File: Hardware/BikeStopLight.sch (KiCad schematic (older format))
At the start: 63 parts, among them J1 ST-Link, J2 PWR, J3 BAT, J4 Conn_01x01, J5 Conn_01x01, J6 Conn_01x08, Q1 NTD4909N, U1 MCP1703A-3302_SOT23, U2 STM32L052K8Tx, U3 RFM95W-868S2, Y1 ABS07-120-32.768KHZ-T

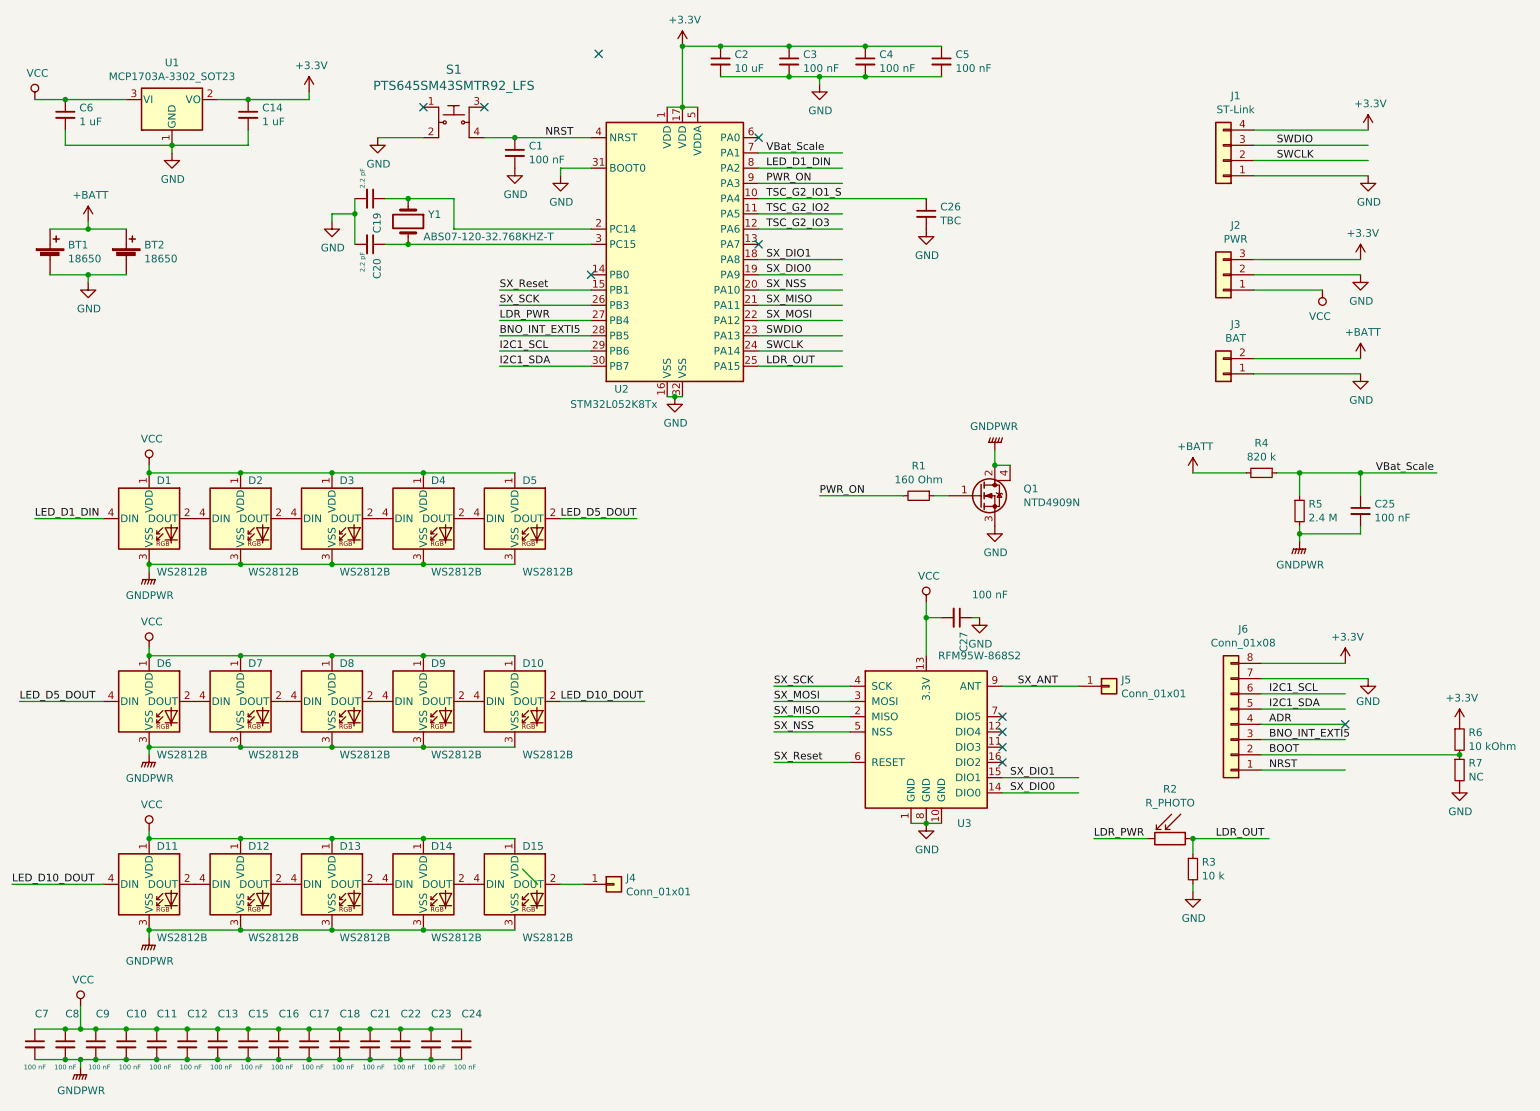
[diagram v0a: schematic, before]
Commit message: WIP - Routed
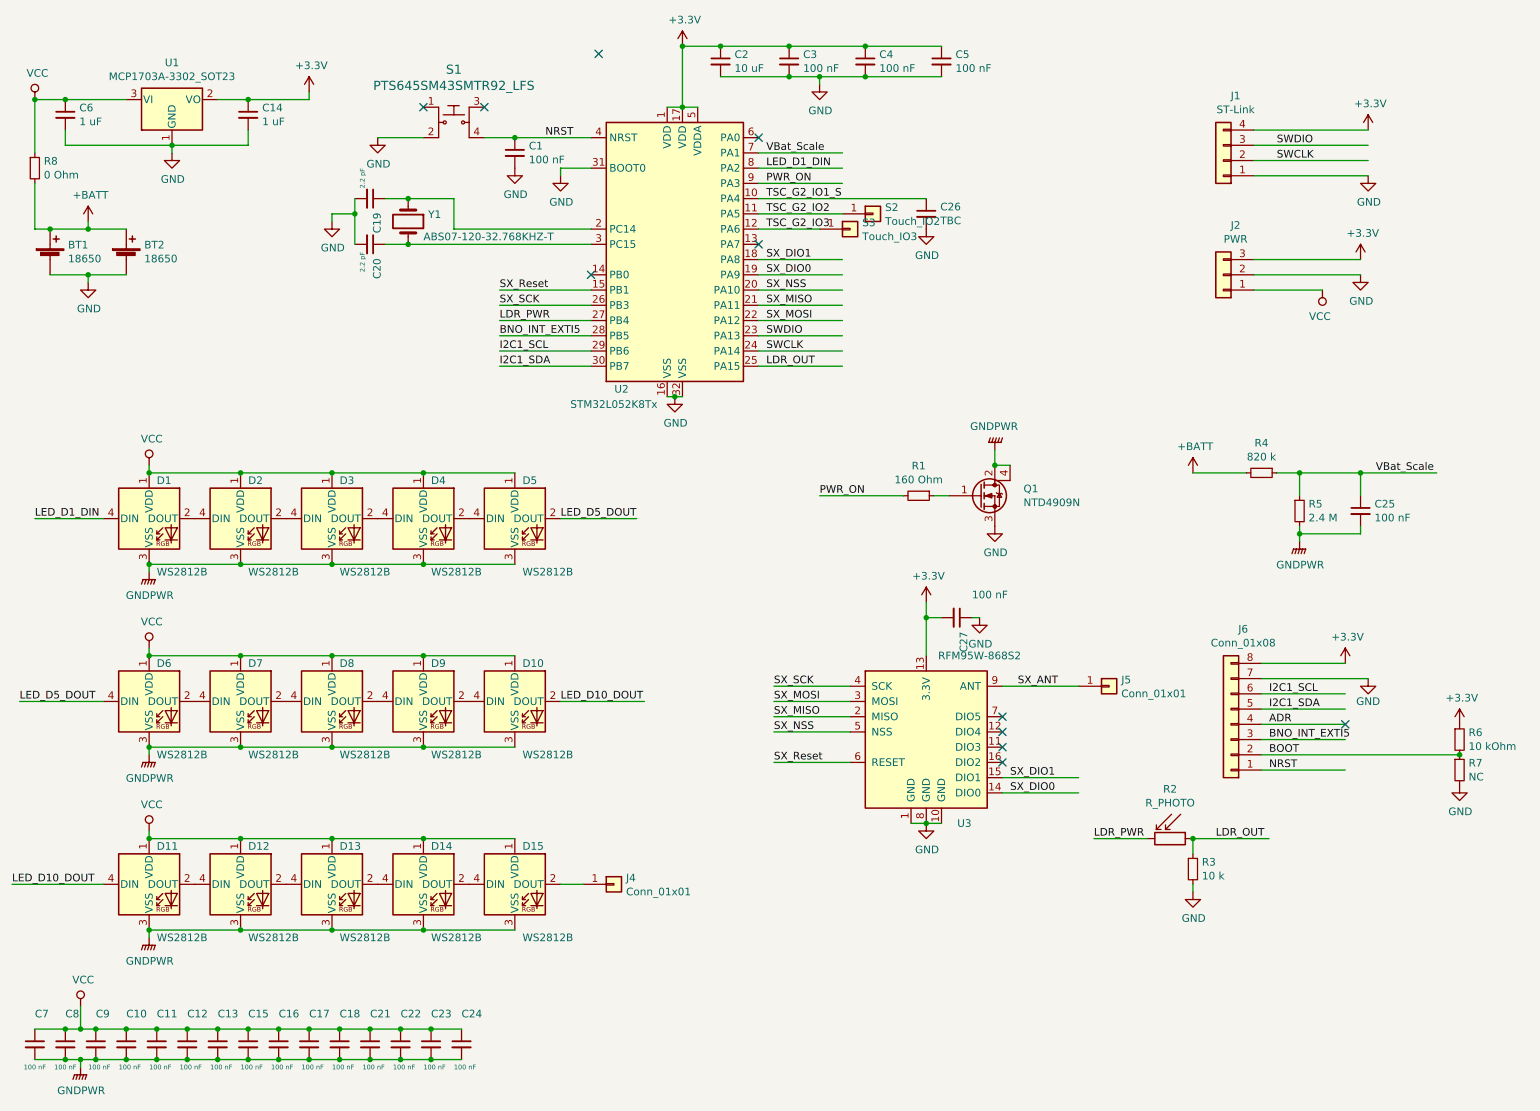
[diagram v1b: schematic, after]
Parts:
- removed J3: BAT, Connector_PinHeader_2.54mm:PinHeader_1x02_P2.54mm_Vertical, symbol Connector_Generic:Conn_01x02
- added R8: 0 Ohm, Resistor_SMD:R_0805_2012Metric, symbol Device:R_Small
- added S2: Touch_IO2, symbol Connector_Generic:Conn_01x01
- added S3: Touch_IO3, symbol Connector_Generic:Conn_01x01
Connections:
- wire segments 182 -> 183
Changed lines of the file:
@@
 Wire Wire Line
 	1100 2250 1350 2250
-$Comp
-L Connector_Generic:Conn_01x02 J3
-U 1 1 5CD40FA1
-P 8550 2900
-F 0 "J3" H 8470 2575 50  0000 C CNN
-F 1 "BAT" H 8470 2666 50  0000 C CNN
-F 2 "Connector_PinHeader_2.54mm:PinHeader_1x02_P2.54mm_Vertical" H 8550 2900 50  0001 C CNN
-F 3 "~" H 8550 2900 50  0001 C CNN
-	1    8550 2900
-	-1   0    0    1
-$EndComp
-Wire Wire Line
-	8750 2900 9450 2900
-Wire Wire Line
-	9450 2800 8750 2800
-$Comp
-L power:+BATT #PWR0108
-U 1 1 5CD4BED2
-P 9450 2800
-F 0 "#PWR0108" H 9450 2650 50  0001 C CNN
-F 1 "+BATT" H 9465 2973 50  0000 C CNN
-F 2 "" H 9450 2800 50  0001 C CNN
-F 3 "" H 9450 2800 50  0001 C CNN
-	1    9450 2800
-	1    0    0    -1
-$EndComp
 Wire Wire Line
 	950  7400 1050 7400
@@
 	1    0    0    -1
 $EndComp
-Entry Wire Line
-	3950 6150 4050 6250
 Wire Wire Line
 	7050 3500 7150 3500
@@
 F 3 "http://www.hoperf.com/upload/rf/RFM95_96_97_98W.pdf" H 3300 6900 50  0001 C CNN
 	1    6600 5250
-	1    0    0    -1
-$EndComp
-$Comp
-L power:VCC #PWR0118
-U 1 1 5CD44CB6
-P 6600 4400
-F 0 "#PWR0118" H 6600 4250 50  0001 C CNN
-F 1 "VCC" H 6617 4573 50  0000 C CNN
-F 2 "" H 6600 4400 50  0001 C CNN
-F 3 "" H 6600 4400 50  0001 C CNN
-	1    6600 4400
 	1    0    0    -1
 $EndComp
@@
 	5500 1850 6050 1850
 Wire Wire Line
-	6050 1950 5500 1950
-Wire Wire Line
 	5500 2350 6050 2350
 Wire Wire Line
@@
 	2700 1900 2700 1850
 $Comp
-L power:GND #PWR0107
-U 1 1 5CE8B7EE
-P 9450 2900
-F 0 "#PWR0107" H 9450 2650 50  0001 C CNN
-F 1 "GND" H 9455 2727 50  0000 C CNN
-F 2 "" H 9450 2900 50  0001 C CNN
-F 3 "" H 9450 2900 50  0001 C CNN
-	1    9450 2900
-	1    0    0    -1
-$EndComp
+L power:+3.3V #PWR0118
+U 1 1 5CE124DA
+P 6600 4400
+F 0 "#PWR0118" H 6600 4250 50  0001 C CNN
+F 1 "+3.3V" H 6615 4573 50  0000 C CNN
+F 2 "" H 6600 4400 50  0001 C CNN
+F 3 "" H 6600 4400 50  0001 C CNN
+	1    6600 4400
+	1    0    0    -1
+$EndComp
+$Comp
+L Device:R_Small R8
+U 1 1 5CE13172
+P 750 1550
+F 0 "R8" H 809 1596 50  0000 L CNN
+F 1 "0 Ohm" H 809 1505 50  0000 L CNN
+F 2 "Resistor_SMD:R_0805_2012Metric" H 750 1550 50  0001 C CNN
+F 3 "~" H 750 1550 50  0001 C CNN
+	1    750  1550
+	1    0    0    -1
+$EndComp
+Wire Wire Line
+	750  1450 750  1100
+Connection ~ 750  1100
+Wire Wire Line
+	750  1650 750  1950
+Wire Wire Line
+	750  1950 850  1950
+Connection ~ 850  1950
+$Comp
+L Connector_Generic:Conn_01x01 S2
+U 1 1 5CE3D1CA
+P 6250 1850
+F 0 "S2" H 6330 1892 50  0000 L CNN
+F 1 "Touch_IO2" H 6330 1801 50  0000 L CNN
+F 2 "" H 6250 1850 50  0001 C CNN
+F 3 "~" H 6250 1850 50  0001 C CNN
+	1    6250 1850
+	1    0    0    -1
+$EndComp
+$Comp
+L Connector_Generic:Conn_01x01 S3
+U 1 1 5CE3D3C0
+P 6100 1950
+F 0 "S3" H 6180 1992 50  0000 L CNN
+F 1 "Touch_IO3" H 6180 1901 50  0000 L CNN
+F 2 "" H 6100 1950 50  0001 C CNN
+F 3 "~" H 6100 1950 50  0001 C CNN
+	1    6100 1950
+	1    0    0    -1
+$EndComp
+Wire Wire Line
+	5500 1950 5900 1950
 $EndSCHEMATC
